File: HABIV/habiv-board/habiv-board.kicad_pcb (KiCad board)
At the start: 4 copper layers, 100.3 x 120.9 mm, 128 parts, among them IC1 RTC_PCF8523T, J1 Micro_SD_Card_Det, J10 Conn_01x02_Female, J11 Conn_01x02_Female, J12 Conn_01x02_Female, J13 Conn_01x02_Female, J14 Conn_01x02_Female, J15 Conn_01x02_Female, J16 Conn_01x02_Female, J17 Conn_01x03_Male, J18 Conn_01x03_Male, J19 Conn_01x03_Male, J2 Conn_ARM_JTAG_SWD_20, J20 Conn_01x05_Male, J21 Conn_01x04_Male, J3 Conn_01x02_Male, J4 Conn_01x16_Male, J5 Conn_01x03_Male, J6 Conn_01x16_Male, J7 Conn_01x16_Male, J8 Conn_01x02_Female, J9 Conn_01x02_Male, Q1 32.768KHz, SW1 SW_DPST_x2, U1 STM32F401RET6, U2 MAX31855, U3 FGPMMOPA6H, U4 TPS564208, U5 TPS564208, U6 LSM9DS1TR, U7 MS560702BA03-00, Y1 32.768MHz

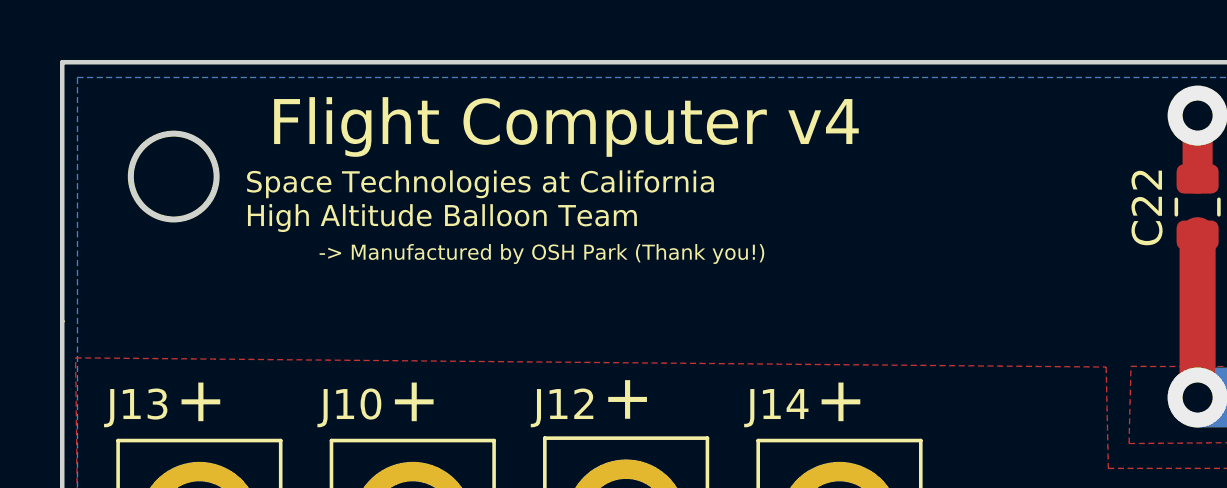
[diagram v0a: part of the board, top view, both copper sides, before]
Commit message: gen stencil
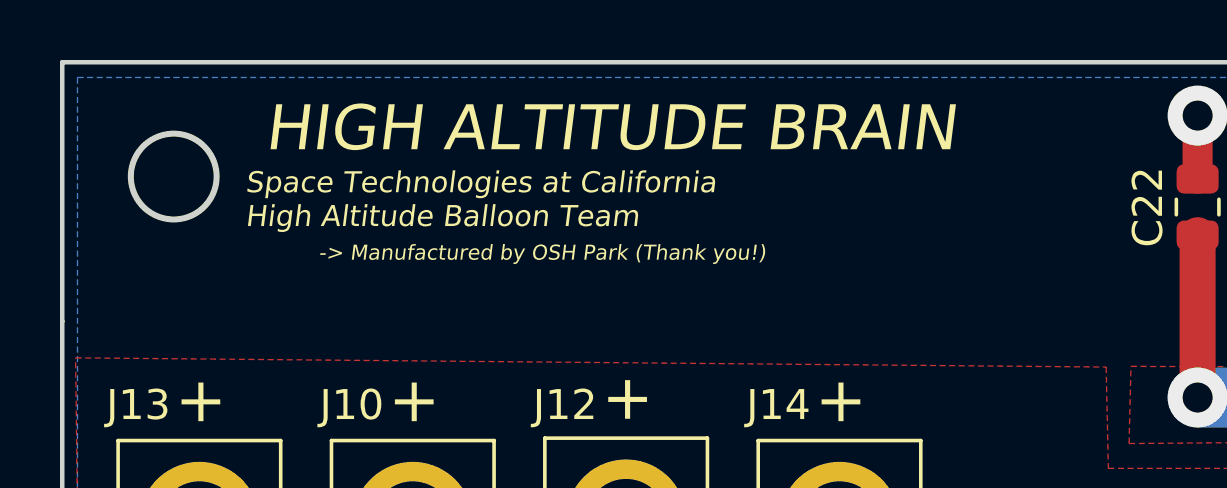
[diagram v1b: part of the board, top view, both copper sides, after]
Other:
- board text added: "HIGH ALTITUDE BRAIN"
- board text removed: "Flight Computer v4"
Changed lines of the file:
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@@
     )
   )
-  (gr_text "Flight Computer v4" (at 97.79 11.176) (layer F.SilkS)
-    (effects (font (size 1.5 1.5) (thickness 0.3)))
+  (gr_text "HIGH ALTITUDE BRAIN" (at 99.3 11.35) (layer F.SilkS)
+    (effects (font (size 1.5 1.5) (thickness 0.3) italic))
   )
   (gr_text "Space Technologies at California\nHigh Altitude Balloon Team" (at 87.122 13.716) (layer F.SilkS)
-    (effects (font (size 0.7 0.7) (thickness 0.1)) (justify left))
+    (effects (font (size 0.7 0.7) (thickness 0.1) italic) (justify left))
   )
   (gr_circle (center 177.706 12.86) (end 179.136 12.86) (layer Edge.Cuts) (width 0.2))
   (gr_text "-> Manufactured by OSH Park (Thank you!)" (at 97.028 15.494) (layer F.SilkS)
-    (effects (font (size 0.5 0.5) (thickness 0.1)))
+    (effects (font (size 0.5 0.5) (thickness 0.1) italic))
   )
   (gr_text Altimeter (at 102.87 96.52) (layer F.SilkS)
